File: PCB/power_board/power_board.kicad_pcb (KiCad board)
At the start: 2 copper layers, 70 x 70 mm, 57 parts, among them IC10 LSM6DSV16BXTR, IC11 TPS61032PWP, IC7 BQ51013BRHLR, IC8 TPS63000IDRCRQ1, IC9 MAX17048G+T10, J10 Conn_01x15, J11 Conn_01x15, J7 Conn_01x02, J8 UJ20-C-H-G-MSMT-R-4C-P16-TR, J9 QVAR, Q2 Si2323DDS-T1-GE3, U2 MCP73871-2CA

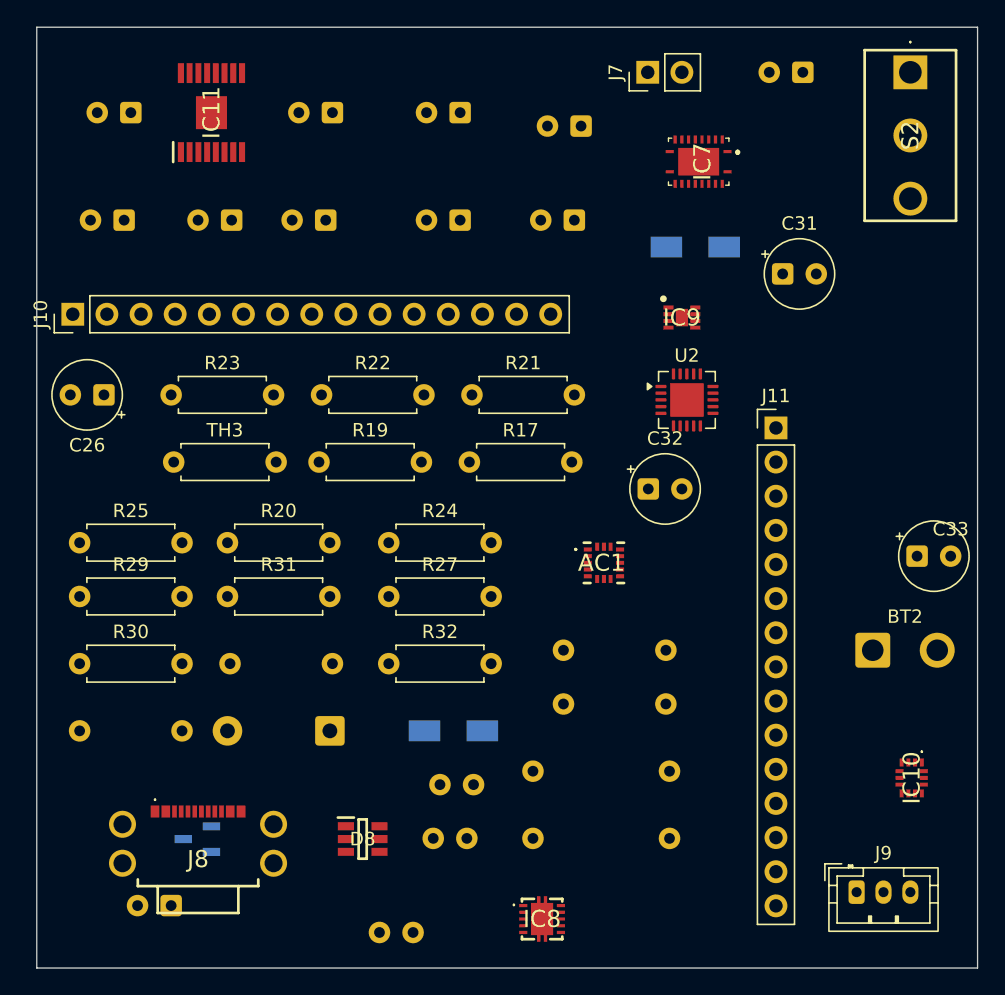
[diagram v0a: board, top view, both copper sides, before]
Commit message: routing done
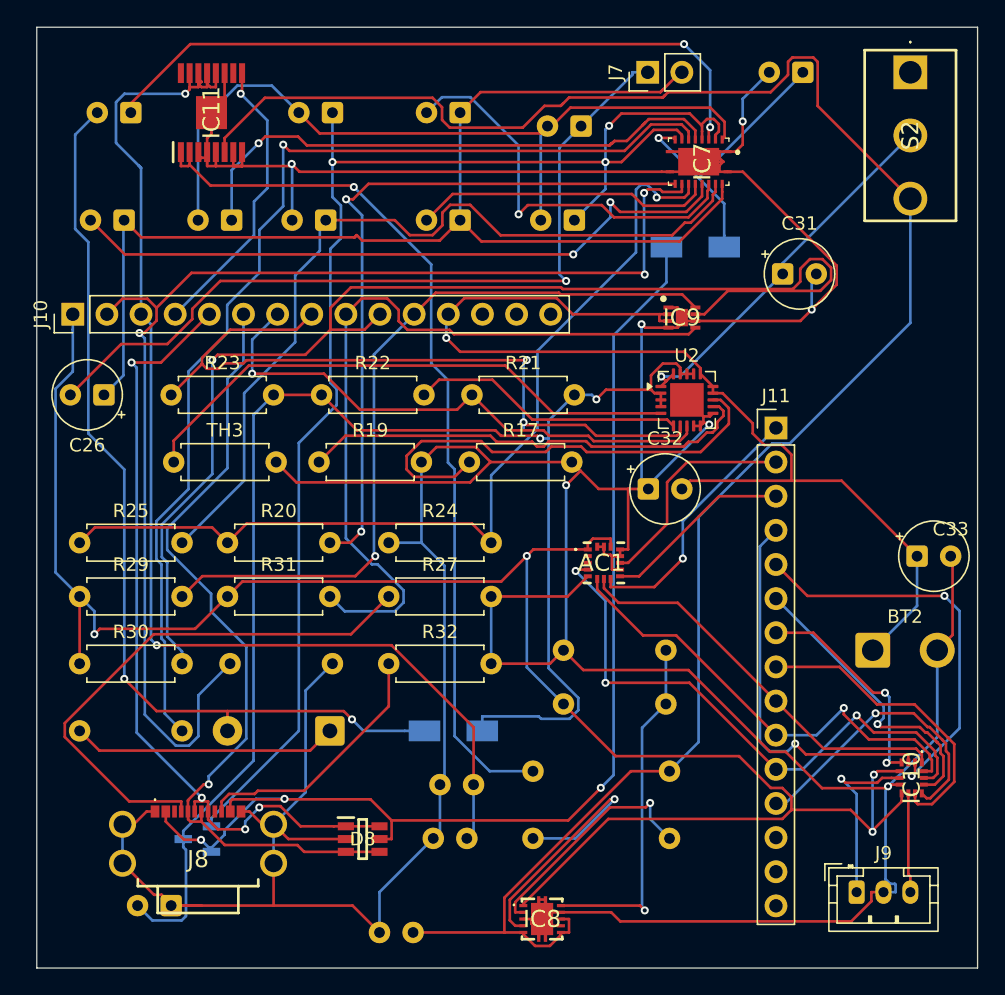
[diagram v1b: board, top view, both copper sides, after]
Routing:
- net GND: track 0.00 -> 393.6 mm, vias 0 -> 7
- net /V_SYS: track 0.00 -> 148.0 mm
- net /Movement/VOUT_3V3: track 0.00 -> 145.4 mm, vias 0 -> 4
- net /CHARGER_SRC: track 0.00 -> 114.6 mm, vias 0 -> 2
- net Net-(IC7-BOOT1): track 0.00 -> 104.9 mm, vias 0 -> 3
- net /TS/CTRL: track 0.00 -> 94.4 mm, vias 0 -> 3
- net /I2C_SCL: track 0.00 -> 92.3 mm, vias 0 -> 1
- net /STEP_UP/OUT+5V: track 0.00 -> 89.3 mm, vias 0 -> 2
- net Net-(IC7-AC2): track 0.00 -> 88.8 mm
- net Net-(D7-A): track 0.00 -> 87.0 mm, vias 0 -> 3
- net /BAT+: track 0.00 -> 81.0 mm, vias 0 -> 1
- net Net-(IC7-~{CHG}): track 0.00 -> 80.3 mm, vias 0 -> 1
- net Net-(D5-A): track 0.00 -> 69.7 mm, vias 0 -> 2
- net Net-(IC7-FOD): track 0.00 -> 68.9 mm, vias 0 -> 1
- net Net-(IC11-SW_1): track 0.00 -> 66.4 mm, vias 0 -> 1
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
